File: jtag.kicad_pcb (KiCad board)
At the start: 4 copper layers, 38.1 x 17.8 mm, 37 parts, among them J9001 USB, J9002 Conn_01x03, J9003 JTAG, P9001 DEBUG/PROG, SW9001 DFU, U9001 LD1117S33TR, U9002 STM32F105RBTx, U9003 74LVCH2T45DC, U9004 74LVCH2T45DC, U9005 74LVCH2T45DC

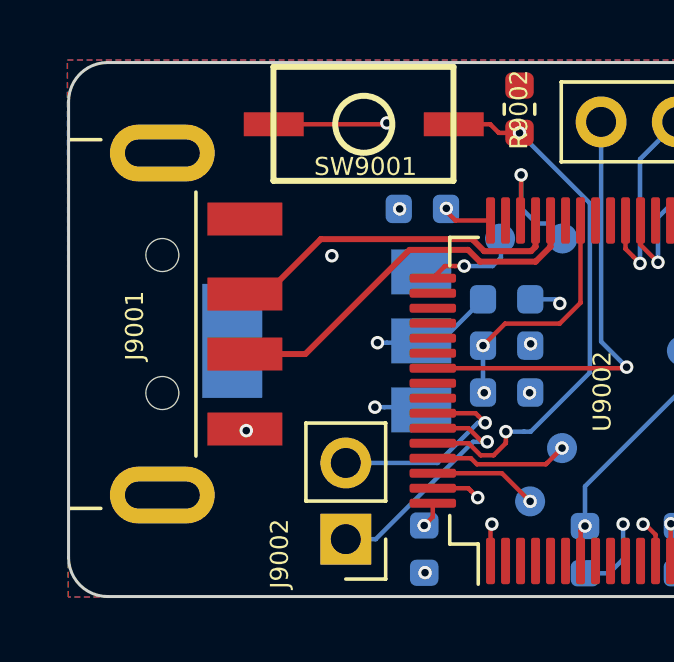
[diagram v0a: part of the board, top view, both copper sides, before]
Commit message: [enhancement] global cleanup
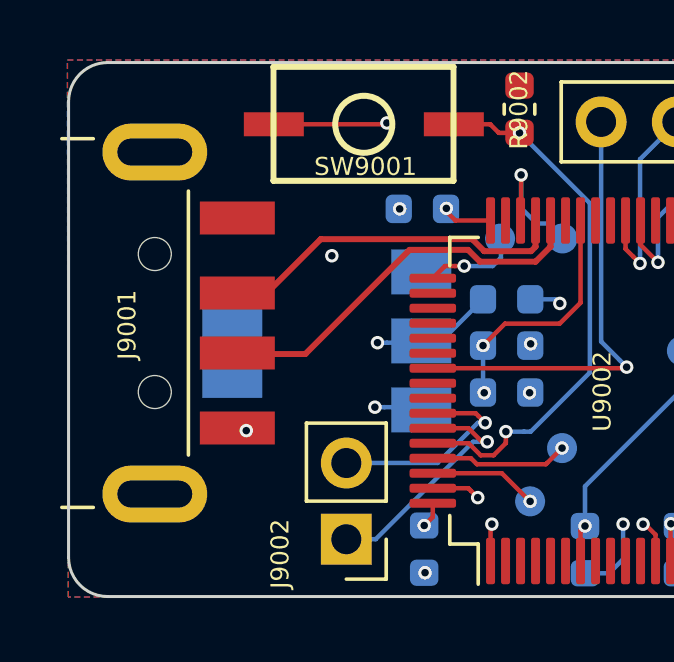
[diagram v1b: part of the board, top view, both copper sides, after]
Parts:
- moved J9001 0.25 mm to (96.3, 44.5)
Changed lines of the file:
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@@
-(kicad_pcb (version 20171130) (host pcbnew "(5.1.0-rc1-8-gc568fadec)")
+(kicad_pcb (version 20171130) (host pcbnew "(5.1.2-1)-1")
   (general
     (thickness 1.6)
@@
   )
   (module Connector_PinHeader_2.54mm:PinHeader_1x02_P2.54mm_Vertical (layer F.Cu)
-    (at 109.57052 51.7455 180)
+    (at 109.5883 51.74742 180)
     (descr "Through hole straight pin header, 1x02, 2.54mm pitch, single row")
     (tags "Through hole pin header THT 1x02 2.54mm single row")
@@
     (pad 2 smd rect (at 0.01631 -3.010692) (size 2 0.8) (layers F.Cu F.Paste F.Mask)
       (net 17 /BOOT0))
-    (model ../../libs/3D/KSR231.wrl
+    (model ${KIPRJMOD}/libs/3D/KSR231.wrl
       (at (xyz 0 0 0))
       (scale (xyz 0.45 0.45 0.45))
@@
   )
   (module Connector_USB:USB_A_CNCTech_1001-011-01101_Horizontal (layer F.Cu)
-    (at 96.55556 44.57446 180)
+    (at 96.3041 44.54144 180)
     (descr http://cnctech.us/pdfs/1001-011-01101.pdf)
     (tags USB-A)
@@
       (rotate (xyz 0 0 0))
     )
+    (model ${KIPRJMOD}/libs/3D/1001-011-01101.stp
+      (offset (xyz 10.7 0 0))
+      (scale (xyz 1 1 1))
+      (rotate (xyz 180 0 90))
+    )
   )
   (module LED_SMD:LED_0603_1608Metric_Castellated (layer F.Cu)
@@
   (gr_line (start 138.43 37.15796) (end 138.43 52.35796) (layer Edge.Cuts) (width 0.1))
   (gr_line (start 101.63 35.85796) (end 137.13 35.85796) (layer Edge.Cuts) (width 0.1))
-  (via (at 114.1857 46.86554) (size 0.45) (drill 0.25) (layers F.Cu B.Cu) (net 2))
-  (via (at 106.25328 48.12792) (size 0.45) (drill 0.25) (layers F.Cu B.Cu) (net 2))
   (via (at 115.697 46.86554) (size 0.45) (drill 0.25) (layers F.Cu B.Cu) (net 1))
   (via (at 115.73256 45.23486) (size 0.45) (drill 0.25) (layers F.Cu B.Cu) (net 1))
-  (via (at 128.15316 51.0286) (size 0.45) (drill 0.25) (layers F.Cu B.Cu) (net 3))
   (via (at 131.81838 49.52492) (size 0.45) (drill 0.25) (layers F.Cu B.Cu) (net 1))
   (via (at 131.826 45.76064) (size 0.45) (drill 0.25) (layers F.Cu B.Cu) (net 1))
   (via (at 131.826 43.71848) (size 0.45) (drill 0.25) (layers F.Cu B.Cu) (net 1))
   (via (at 125.68936 45.81652) (size 0.45) (drill 0.25) (layers F.Cu B.Cu) (net 1))
-  (via (at 125.72746 51.1048) (size 0.45) (drill 0.25) (layers F.Cu B.Cu) (net 3))
   (via (at 125.68936 49.51476) (size 0.45) (drill 0.25) (layers F.Cu B.Cu) (net 1))
   (via (at 122.44832 40.91178) (size 0.45) (drill 0.25) (layers F.Cu B.Cu) (net 1))
@@
   (segment (start 119.89556 51.59758) (end 119.54502 51.24704) (width 0.15) (layer F.Cu) (net 1))
   (segment (start 119.54502 51.24704) (end 119.47906 51.24704) (width 0.15) (layer F.Cu) (net 1))
+  (via (at 114.1857 46.86554) (size 0.45) (drill 0.25) (layers F.Cu B.Cu) (net 2))
+  (via (at 106.25328 48.12792) (size 0.45) (drill 0.25) (layers F.Cu B.Cu) (net 2))
   (segment (start 114.14496 45.29328) (end 114.14496 46.85792) (width 0.15) (layer B.Cu) (net 2))
   (segment (start 117.39556 41.12258) (end 117.39556 43.8665) (width 0.15) (layer F.Cu) (net 2))
@@
   (segment (start 111.978 47.3456) (end 110.858998 47.3456) (width 0.15) (layer B.Cu) (net 2))
   (segment (start 110.858998 47.3456) (end 110.5408 47.3456) (width 0.15) (layer B.Cu) (net 2))
+  (via (at 128.15316 51.0286) (size 0.45) (drill 0.25) (layers F.Cu B.Cu) (net 3))
+  (via (at 125.72746 51.1048) (size 0.45) (drill 0.25) (layers F.Cu B.Cu) (net 3))
   (via (at 112.18418 51.29012) (size 0.45) (drill 0.25) (layers F.Cu B.Cu) (net 3))
   (segment (start 112.47056 51.00374) (end 112.18418 51.29012) (width 0.15) (layer F.Cu) (net 3))

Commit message: [enhancement] move pcb screenshots to imgs directory
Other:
- board text added: "The current 4 layer 1.6mm board stackup is as follows: Thickness Layer ======================================== 0.0356mm copper 0.1702mm FR408 prepreg 0.0178mm copper 1.1938mm FR408 0.0178mm copper 0.1702mm FR408 prepreg 0.0356mm copper 0.0254mm solder resist"
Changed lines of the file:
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@@
   (general
     (thickness 1.6)
-    (drawings 8)
+    (drawings 9)
     (tracks 355)
     (zones 0)
@@
     )
   )
+  (gr_text "The current 4 layer 1.6mm board stackup is as follows:\n\nThickness           Layer\n========================================\n0.0356mm       copper\n0.1702mm       FR408 prepreg\n0.0178mm       copper\n1.1938mm       FR408 \n0.0178mm       copper\n0.1702mm       FR408 prepreg\n0.0356mm       copper\n0.0254mm       solder resist" (at 89.2429 79.29626) (layer Cmts.User)
+    (effects (font (size 1.5 1.5) (thickness 0.3)) (justify left))
+  )
   (gr_arc (start 137.13 52.35796) (end 138.43 52.35796) (angle 90) (layer Edge.Cuts) (width 0.1))
